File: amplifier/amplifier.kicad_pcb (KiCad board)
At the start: 2 copper layers, 65 x 30 mm, 8 parts

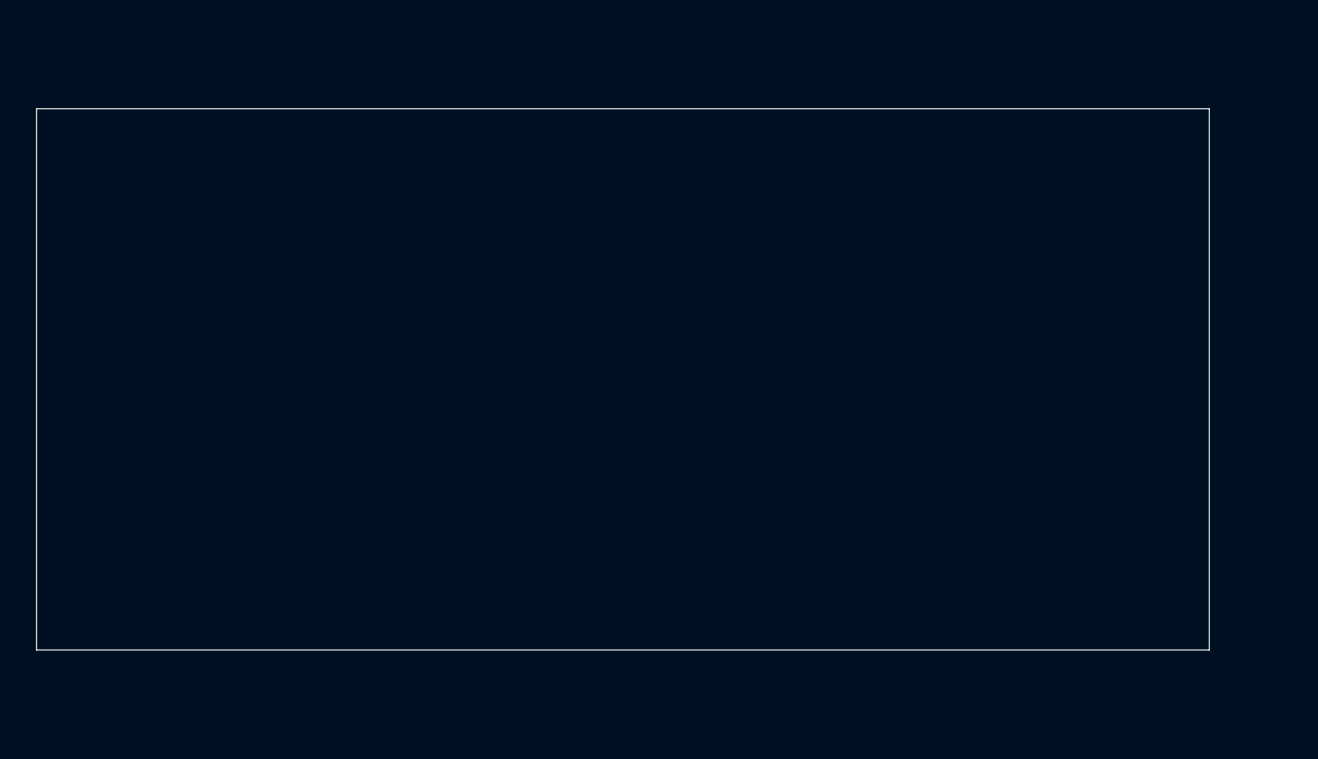
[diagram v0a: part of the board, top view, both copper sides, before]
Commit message: .
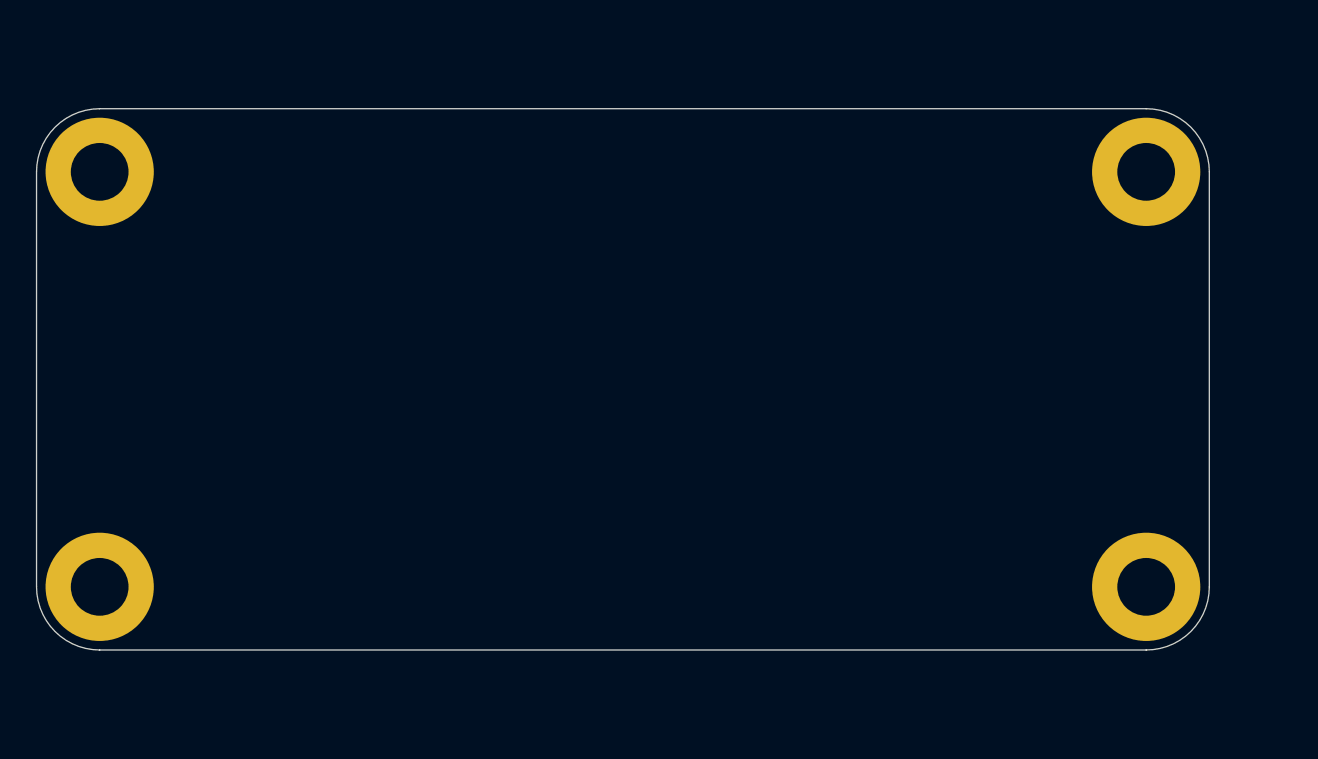
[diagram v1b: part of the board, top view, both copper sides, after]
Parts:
- added H5: MountingHole_M3_3.2mm_Pad, PCM_SL_Mechanical:MountingHole_3.2mm_Pad, F.Cu at (53.5, 53.5)
- added H6: MountingHole_M3_3.2mm_Pad, PCM_SL_Mechanical:MountingHole_3.2mm_Pad, F.Cu at (111.5, 53.5)
- added H7: MountingHole_M3_3.2mm_Pad, PCM_SL_Mechanical:MountingHole_3.2mm_Pad, F.Cu at (53.5, 76.5)
- added H8: MountingHole_M3_3.2mm_Pad, PCM_SL_Mechanical:MountingHole_3.2mm_Pad, F.Cu at (111.5, 76.5)
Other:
- outline, holes or cut-outs redrawn
